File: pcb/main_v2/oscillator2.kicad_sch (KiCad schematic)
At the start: 23 parts, among them IC601 PD0922J5050S2HF, U601 ADF4351

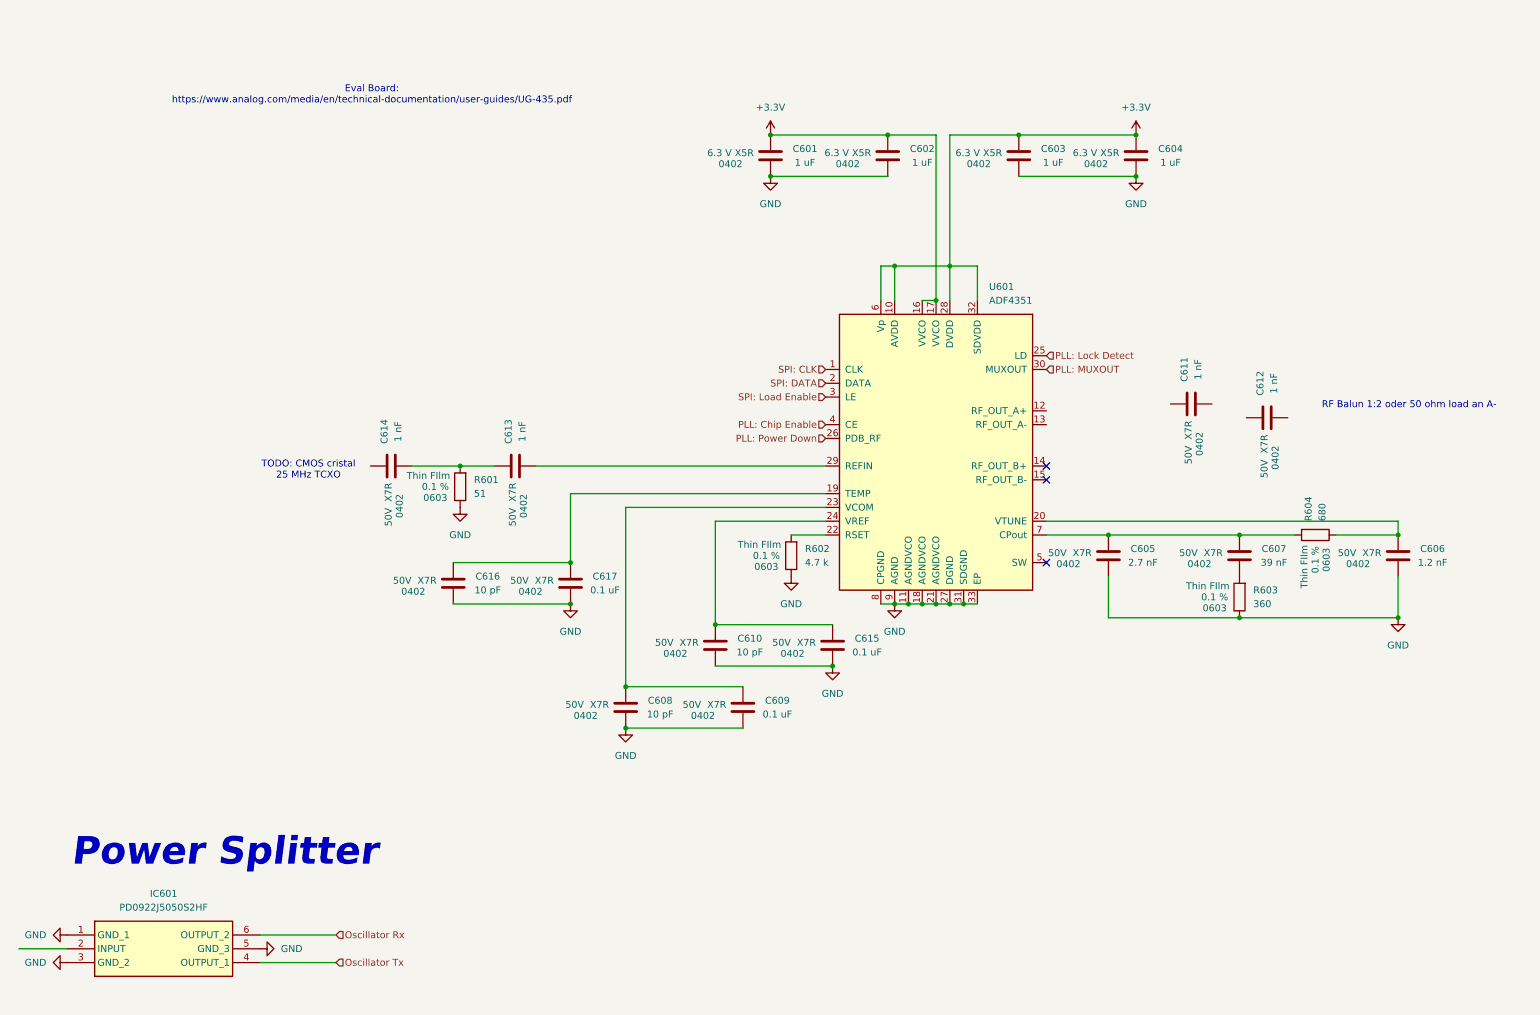
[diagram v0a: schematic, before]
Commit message: updated pll
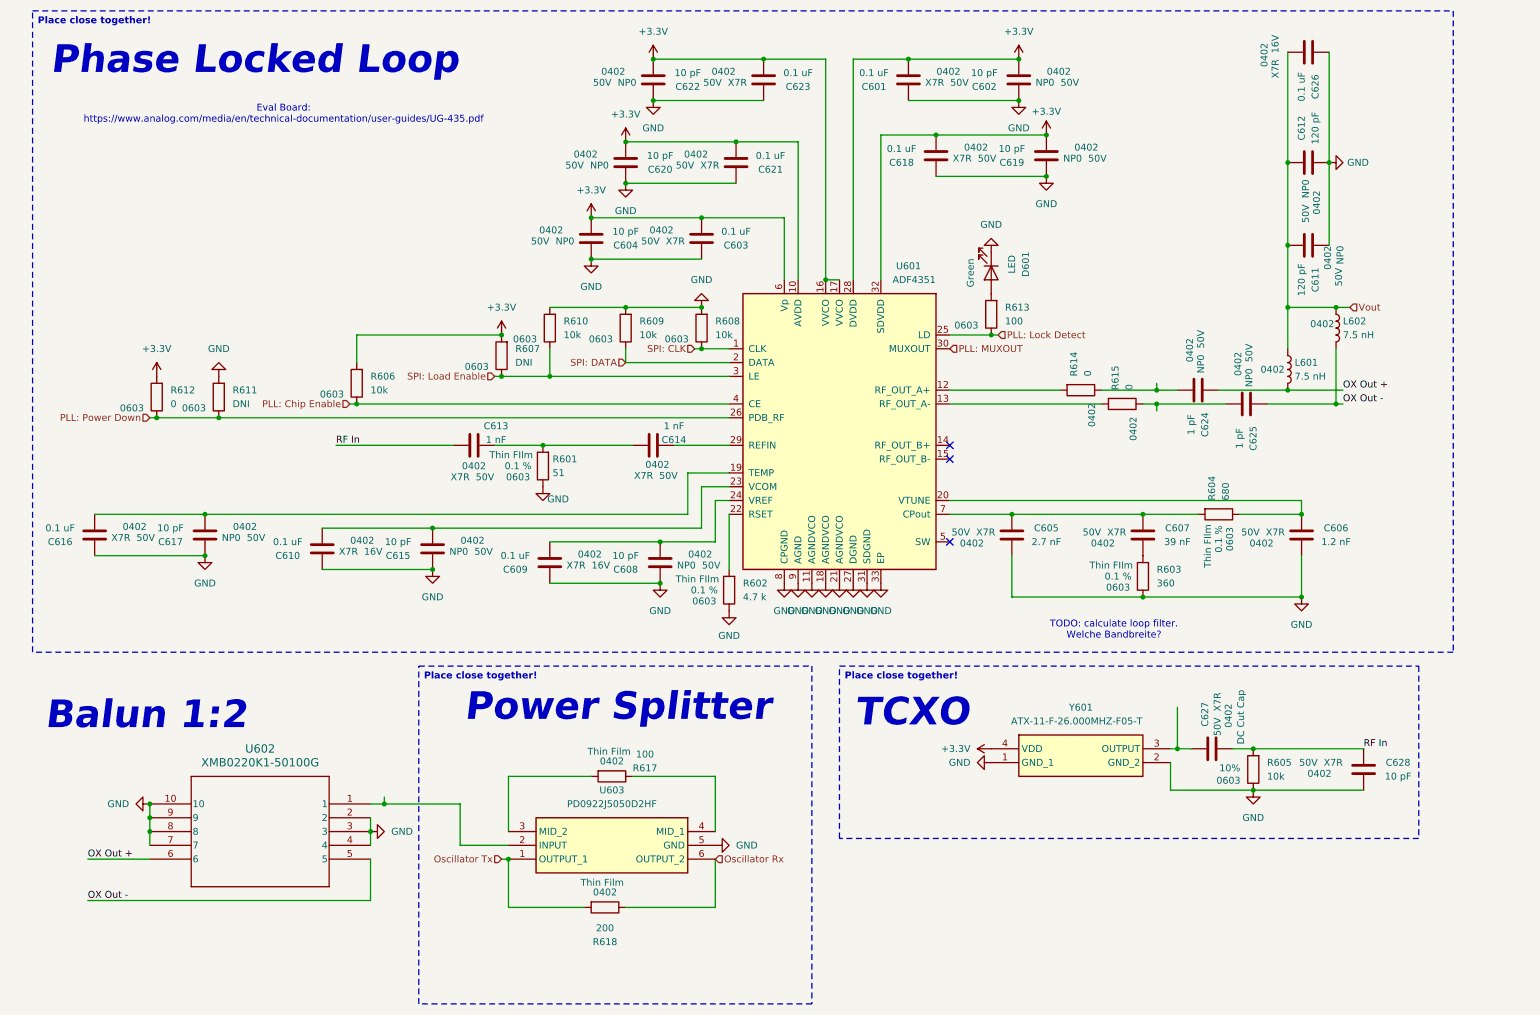
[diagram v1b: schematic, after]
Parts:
- removed IC601: PD0922J5050S2HF, My Footprints:PD0922J5050S2HF, symbol My Symbols:PD0922J5050S2HF
- added C618, C621, C623, C626: 0.1 uF, Capacitor_SMD:C_0402_1005Metric, symbol Device:C
- added C619, C620, C622, C628: 10 pF, Capacitor_SMD:C_0402_1005Metric, symbol Device:C
- added C624, C625: 1 pF, Capacitor_SMD:C_0402_1005Metric, symbol Device:C
- added C627: DC Cut Cap, Capacitor_SMD:C_0402_1005Metric, symbol Device:C
- added D601: LED, LED_SMD:LED_0805_2012Metric, symbol Device:LED
- added L601, L602: 7.5 nH, Inductor_SMD:L_0402_1005Metric, symbol Device:L
- added R605, R606, R608, R609, R610: 10k, Resistor_SMD:R_0603_1608Metric, symbol Device:R
- added R607, R611: DNI, Resistor_SMD:R_0603_1608Metric, symbol Device:R
- added R612, R614, R615: 0, Resistor_SMD:R_0603_1608Metric, symbol Device:R
- added R613: 100, Resistor_SMD:R_0603_1608Metric, symbol Device:R
- added R617: 100, Resistor_SMD:R_0402_1005Metric, symbol Device:R
- added R618: 200, Resistor_SMD:R_0402_1005Metric, symbol Device:R
- added U602: XMB0220K1-50100G, My Footprints:XMB0220K1-50100G_TTT, symbol My Symbols:XMB0220K1-50100G
- added U603: PD0922J5050D2HF, PD0922J5050D2HF, symbol My Symbols:PD0922J5050D2HF
- added Y601: ATX-11-F-26.000MHZ-F05-T, ATX11F26000MHZF05T, symbol My Symbols:ATX-11-F-26.000MHZ-F05-T
- C601, C603: value 1 uF -> 0.1 uF; Material X5R -> X7R; Package 0402 -> 0402; Tolerance 10 % -> ±10%; Voltage 6.3 V -> 50V
- C602, C604: value 1 uF -> 10 pF; Material X5R -> NP0; Package 0402 -> 0402; Tolerance 10 % -> ±10%; Voltage 6.3 V -> 50V
- C608: Material X7R -> NP0
- C609: Voltage 50V -> 16V
- C610: value 10 pF -> 0.1 uF; Voltage 50V -> 16V
- C611, C612: value 1 nF -> 120 pF; Material X7R -> NP0
- C615, C617: value 0.1 uF -> 10 pF; Material X7R -> NP0
- C616: value 10 pF -> 0.1 uF
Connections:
- net +3.3V: now also C601.1, C602.1, C603.1, C604.1, C618.1, C619.1, C620.1, C621.1, C622.1, C623.1, R606.2, R607.2, R612.2, Y601.4 (VDD); no longer C601.2, C602.2, C603.2, C604.2
- net GND: now also C601.2, C602.2, C603.2, C604.2, C608.2, C609.2, C610.2, C611.2, C612.1, C615.2, C616.2, C617.2, C618.2, C619.2, C620.2, C621.2, C622.2, C623.2, C626.2, C628.1, D601.1 (K), R605.1, R608.2, R609.2, R610.2, R611.2, U602.10, U602.2, U602.3, U602.4, U602.7, U602.8, U602.9, U603.5 (GND), Y601.1 (GND_1), Y601.2 (GND_2); no longer C601.1, C602.1, C603.1, C604.1, C608.1, C609.1, C610.1, C615.1, C616.1, C617.1
- net Oscillator Rx: now also R618.1, U603.6 (OUTPUT_2)
- net Oscillator Tx: now also R618.2, U603.1 (OUTPUT_1)
- net PLL: Chip Enable: now also R606.1
- net PLL: Lock Detect: now also R613.1
- net PLL: Power Down: now also R611.1, R612.1
- net SPI: CLK: now also R608.1
- net SPI: DATA: now also R609.1
- net SPI: Load Enable: now also R607.1, R610.1
- net Vout: now reaches C612.2
- net Vout: now also C611.1, C626.1, L601.1, L602.1
- net at U601.12 (RF_OUT_A+): now also R614.2
- net at U601.13 (RF_OUT_A-): now also R615.2
- net at U601.29 (REFIN): now also C614.1; no longer C613.1
- net at C614.2: now also C613.1, R601.2
- new net: C625.1, R615.1
- new net: C616.1, C617.1, U601.19 (TEMP)
- new net: C627.2, Y601.3 (OUTPUT)
- new net: C610.1, C615.1, U601.23 (VCOM)
- new net: C608.1, C609.1, U601.24 (VREF)
- new net: U602.1, U603.2 (INPUT)
- new net: C624.1, R614.1
- new net: D601.2 (A), R613.2
- new net: R617.1, U603.4 (MID_1)
- new net: R617.2, U603.3 (MID_2)
- new net OX Out +: C624.2, L601.2, U602.6
- new net OX Out -: C625.2, L602.2, U602.5
- new net RF In: C613.2, C627.1, C628.2, R605.2
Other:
- note added: "Balun 1:2"
- note added: "Phase Locked Loop"
- note added: "TCXO"
- note added: "TODO: calculate loop filter. Welche Bandbreite?"
- note removed: "RF Balun 1:2 oder 50 ohm load an A-"
- note removed: "TODO: CMOS cristal 25 MHz TCXO"
- moved on the sheet: C605, C606, C607, R602, R603, R604, U601
